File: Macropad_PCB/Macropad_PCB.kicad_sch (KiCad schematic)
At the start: 0 parts

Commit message: Project init
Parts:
- added SW1: SW_Push, Button_Switch_Keyboard:SW_Cherry_MX_1.00u_PCB, symbol Switch:SW_Push
- added SW2: RotaryEncoder, Rotary_Encoder:RotaryEncoder_Alps_EC11E-Switch_Vertical_H20mm, symbol Device:RotaryEncoder
- added U1: MOUDLE-SEEEDUINO-XIAO, footprints:XIAO-Generic-Hybrid-14P-2.54-21X17.8MM, symbol XIAO_RP2040:MOUDLE-SEEEDUINO-XIAO
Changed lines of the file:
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@@
 	(generator_version "9.0")
 	(paper "A4")
+	(symbol
+		(lib_id "Device:RotaryEncoder")
+		(at 157.48 24.13 0)
+		(unit 1)
+		(exclude_from_sim no)
+		(in_bom yes)
+		(on_board yes)
+		(dnp no)
+		(fields_autoplaced yes)
+		(property "Reference" "SW2"
+			(at 163.83 22.8599 0)
+			(effects
+				(font
+					(size 1.27 1.27)
+				)
+				(justify left)
+			)
+		)
+		(property "Value" "RotaryEncoder"
+			(at 163.83 25.3999 0)
+			(effects
+				(font
+					(size 1.27 1.27)
+				)
+				(justify left)
+			)
+		)
+		(property "Footprint" "Rotary_Encoder:RotaryEncoder_Alps_EC11E-Switch_Vertical_H20mm"
+			(at 153.67 20.066 0)
+			(effects
+				(font
+					(size 1.27 1.27)
+				)
+				(hide yes)
+			)
+		)
+		(property "Datasheet" "~"
+			(at 157.48 17.526 0)
+			(effects
+				(font
+					(size 1.27 1.27)
+				)
+				(hide yes)
+			)
+		)
+		(property "Description" "Rotary encoder, dual channel, incremental quadrate outputs"
+			(at 157.48 24.13 0)
+			(effects
+				(font
+					(size 1.27 1.27)
+				)
+				(hide yes)
+			)
+		)
+		(pin "B"
+		)
+		(pin "A"
+		)
+		(pin "C"
+		)
+		(instances
+			(project ""
+				(path "/1a1a6edd-d890-43f8-a81d-660412c01a38"
+					(reference "SW2")
+					(unit 1)
+				)
+			)
+		)
+	)
+	(symbol
+		(lib_id "XIAO_RP2040:MOUDLE-SEEEDUINO-XIAO")
+		(at 74.93 30.48 0)
+		(unit 1)
+		(exclude_from_sim no)
+		(in_bom yes)
+		(on_board yes)
+		(dnp no)
+		(fields_autoplaced yes)
+		(property "Reference" "U1"
+			(at 76.2 15.24 0)
+			(effects
+				(font
+					(size 1.27 1.27)
+				)
+			)
+		)
+		(property "Value" "MOUDLE-SEEEDUINO-XIAO"
+			(at 76.2 17.78 0)
+			(effects
+				(font
+					(size 1.27 1.27)
+				)
+			)
+		)
+		(property "Footprint" "footprints:XIAO-Generic-Hybrid-14P-2.54-21X17.8MM"
+			(at 58.42 27.94 0)
+			(effects
+				(font
+					(size 1.27 1.27)
+				)
+				(hide yes)
+			)
+		)
+		(property "Datasheet" ""
+			(at 58.42 27.94 0)
+			(effects
+				(font
+					(size 1.27 1.27)
+				)
+				(hide yes)
+			)
+		)
+		(property "Description" ""
+			(at 74.93 30.48 0)
+			(effects
+				(font
+					(size 1.27 1.27)
+				)
+				(hide yes)
+			)
+		)
+		(pin "10"
+		)
+		(pin "6"
+		)
+		(pin "7"
+		)
+		(pin "4"
+		)
+		(pin "14"
+		)
+		(pin "3"
+		)
+		(pin "5"
+		)
+		(pin "9"
+		)
+		(pin "8"
+		)
+		(pin "2"
+		)
+		(pin "12"
+		)
+		(pin "11"
+		)
+		(pin "1"
+		)
+		(pin "13"
+		)
+		(instances
+			(project ""
+				(path "/1a1a6edd-d890-43f8-a81d-660412c01a38"
+					(reference "U1")
+					(unit 1)
+				)
+			)
+		)
+	)
+	(symbol
+		(lib_id "Switch:SW_Push")
+		(at 92.71 69.85 0)
+		(unit 1)
+		(exclude_from_sim no)
+		(in_bom yes)
+		(on_board yes)
+		(dnp no)
+		(fields_autoplaced yes)
+		(property "Reference" "SW1"
+			(at 92.71 62.23 0)
+			(effects
+				(font
+					(size 1.27 1.27)
+				)
+			)
+		)
+		(property "Value" "SW_Push"
+			(at 92.71 64.77 0)
+			(effects
+				(font
+					(size 1.27 1.27)
+				)
+			)
+		)
+		(property "Footprint" "Button_Switch_Keyboard:SW_Cherry_MX_1.00u_PCB"
+			(at 92.71 64.77 0)
+			(effects
+				(font
+					(size 1.27 1.27)
+				)
+				(hide yes)
+			)
+		)
+		(property "Datasheet" "~"
+			(at 92.71 64.77 0)
+			(effects
+				(font
+					(size 1.27 1.27)
+				)
+				(hide yes)
+			)
+		)
+		(property "Description" "Push button switch, generic, two pins"
+			(at 92.71 69.85 0)
+			(effects
+				(font
+					(size 1.27 1.27)
+				)
+				(hide yes)
+			)
+		)
+		(pin "1"
+		)
+		(pin "2"
+		)
+		(instances
+			(project ""
+				(path "/1a1a6edd-d890-43f8-a81d-660412c01a38"
+					(reference "SW1")
+					(unit 1)
+				)
+			)
+		)
+	)
 	(sheet_instances
 		(path "/"

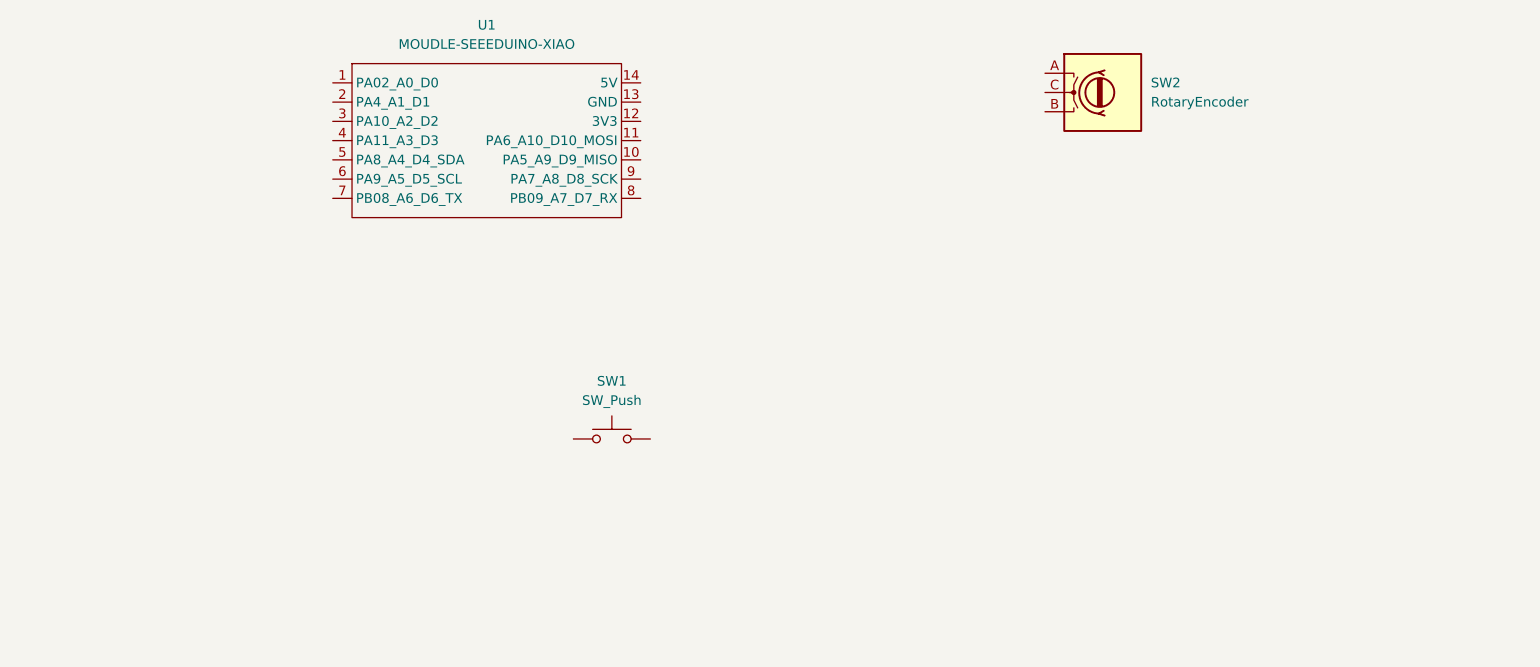
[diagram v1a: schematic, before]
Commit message: Inizio PCB
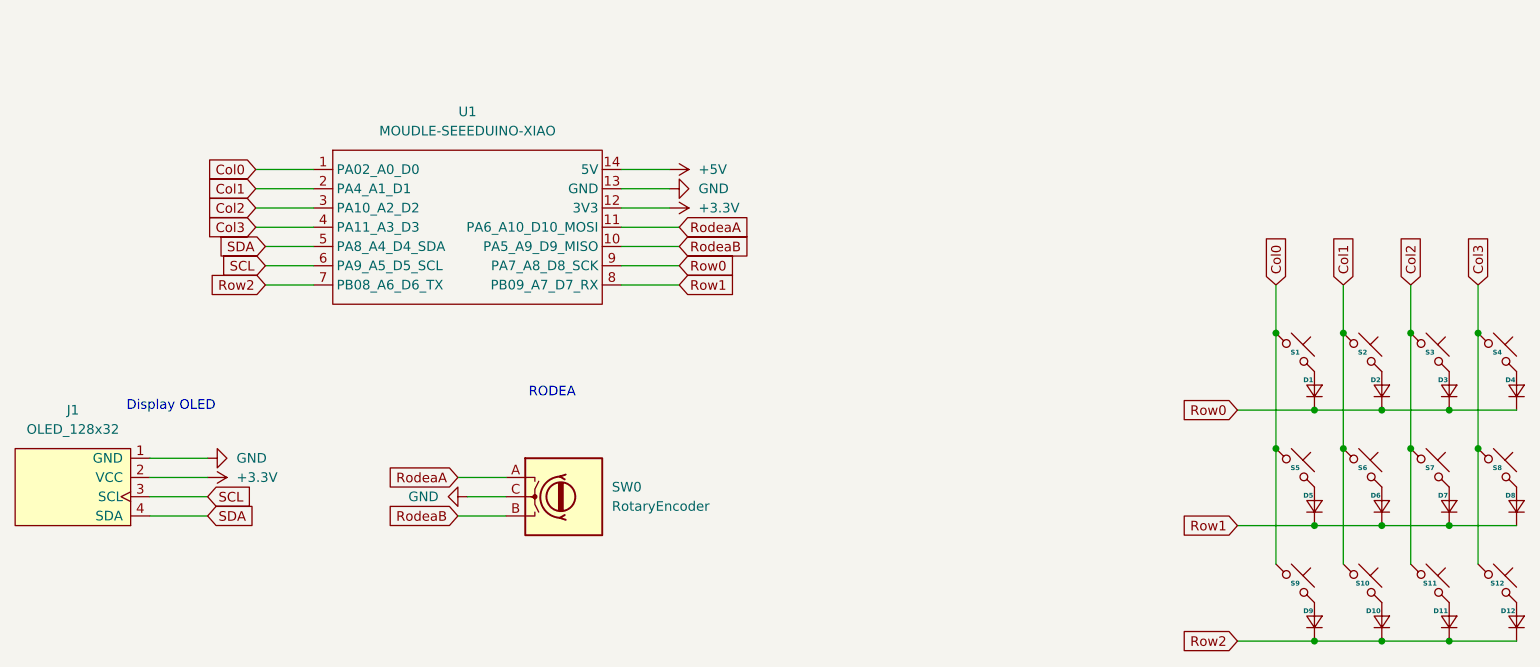
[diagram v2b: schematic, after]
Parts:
- removed SW1: SW_Push, Button_Switch_Keyboard:SW_Cherry_MX_1.00u_PCB, symbol Switch:SW_Push
- added D1, D10, D11, D12, D2, D3, D4, D5, D6, D7, D8, D9: ~, ScottoKeebs_Components:Diode_DO-35, symbol ScottoKeebs:Placeholder_Diode
- added J1: OLED_128x32, ScottoKeebs_Components:OLED_128x32, symbol ScottoKeebs:OLED_128x32
- added S1, S10, S11, S12, S2, S3, S4, S5, S6, S7, S8, S9: ~, ScottoKeebs_MX:MX_PCB_1.00u, symbol ScottoKeebs:Placeholder_Keyswitch
- renumbered SW2 to SW0
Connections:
- net RodeaA: now reaches SW0.A
- net RodeaA: now also U1.11 (PA6_A10_D10_MOSI)
- net RodeaB: now reaches SW0.B
- net RodeaB: now also U1.10 (PA5_A9_D9_MISO)
- net GND: now reaches SW0.C
- net GND: now also U1.13 (GND), J1.1 (GND)
- net Col0: now reaches U1.1 (PA02_A0_D0)
- net Col0: now also S1.1, S5.1, S9.1
- net +3.3V: now reaches U1.12 (3V3)
- net +3.3V: now also J1.2 (VCC)
- net +5V: now reaches U1.14 (5V)
- net Col1: now reaches U1.2 (PA4_A1_D1)
- net Col1: now also S10.1, S2.1, S6.1
- net Col2: now reaches U1.3 (PA10_A2_D2)
- net Col2: now also S11.1, S3.1, S7.1
- net Col3: now reaches U1.4 (PA11_A3_D3)
- net Col3: now also S12.1, S4.1, S8.1
- net SDA: now reaches U1.5 (PA8_A4_D4_SDA)
- net SDA: now also J1.4 (SDA)
- net SCL: now reaches U1.6 (PA9_A5_D5_SCL)
- net SCL: now also J1.3 (SCL)
- net Row2: now reaches U1.7 (PB08_A6_D6_TX)
- net Row2: now also D10.1 (K), D11.1 (K), D12.1 (K), D9.1 (K)
- net Row1: now reaches U1.8 (PB09_A7_D7_RX)
- net Row1: now also D5.1 (K), D6.1 (K), D7.1 (K), D8.1 (K)
- net Row0: now reaches U1.9 (PA7_A8_D8_SCK)
- net Row0: now also D1.1 (K), D2.1 (K), D3.1 (K), D4.1 (K)
- new net: D12.2 (A), S12.2
- new net: D4.2 (A), S4.2
- new net: D3.2 (A), S3.2
- new net: D2.2 (A), S2.2
- new net: D1.2 (A), S1.2
- new net: D6.2 (A), S6.2
- new net: D11.2 (A), S11.2
- new net: D10.2 (A), S10.2
- new net: D9.2 (A), S9.2
- new net: D7.2 (A), S7.2
- new net: D8.2 (A), S8.2
- new net: D5.2 (A), S5.2
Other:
- note added: "Display OLED"
- note added: "RODEA"
- moved on the sheet: SW0, U1

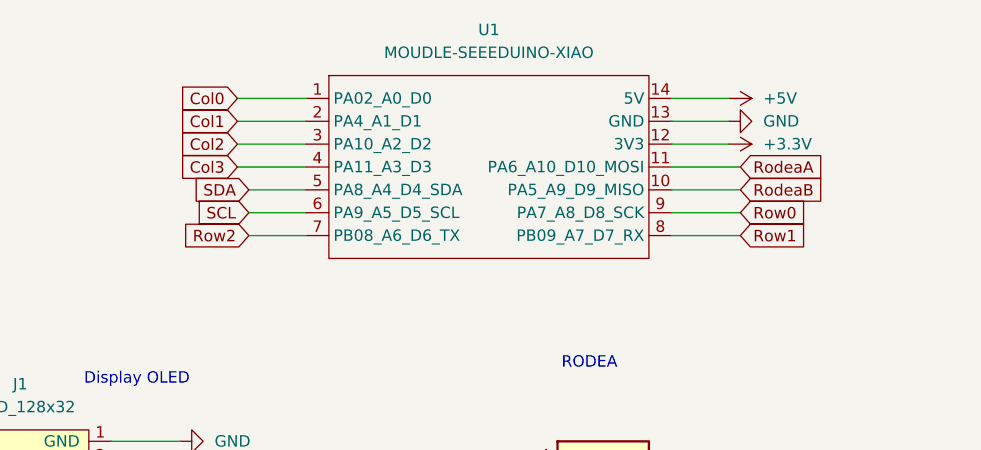
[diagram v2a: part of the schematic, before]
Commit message: PCB. Ancora alcuni errori
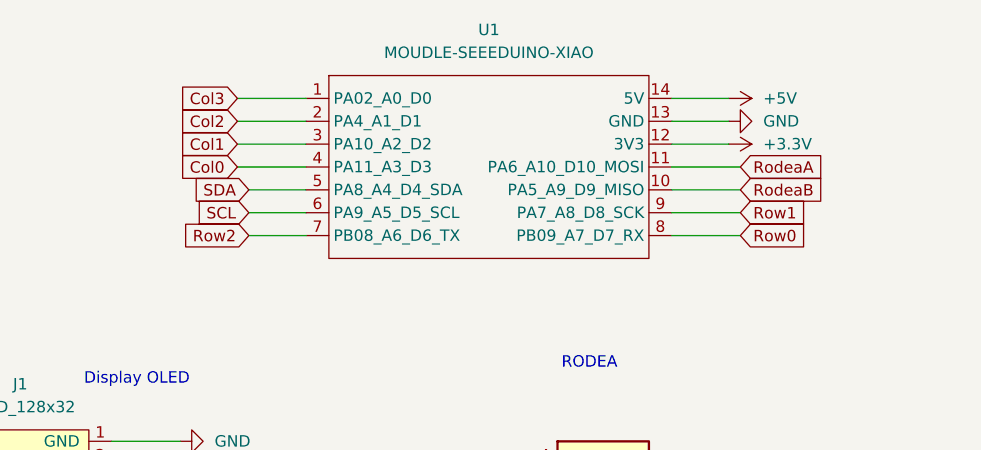
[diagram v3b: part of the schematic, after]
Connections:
- net Col0: now also U1.4 (PA11_A3_D3); no longer U1.1 (PA02_A0_D0)
- net Col1: now also U1.3 (PA10_A2_D2); no longer U1.2 (PA4_A1_D1)
- net Col2: now also U1.2 (PA4_A1_D1); no longer U1.3 (PA10_A2_D2)
- net Col3: now also U1.1 (PA02_A0_D0); no longer U1.4 (PA11_A3_D3)
- net Row0: now also U1.8 (PB09_A7_D7_RX); no longer U1.9 (PA7_A8_D8_SCK)
- net Row1: now also U1.9 (PA7_A8_D8_SCK); no longer U1.8 (PB09_A7_D7_RX)

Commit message: Project exportation
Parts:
- D1, D10, D11, D12, D2, D3, D4, D5, D6, D7, D8, D9: footprint ScottoKeebs_Components:Diode_DO-35 -> Diode_THT:D_DO-35_SOD27_P7.62mm_Horizontal
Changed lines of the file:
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@@
 			)
 		)
-		(property "Footprint" "ScottoKeebs_Components:Diode_DO-35"
+		(property "Footprint" "Diode_THT:D_DO-35_SOD27_P7.62mm_Horizontal"
 			(at 203.2 63.5 90)
 			(effects
@@
 			)
 		)
-		(property "Footprint" "ScottoKeebs_Components:Diode_DO-35"
+		(property "Footprint" "Diode_THT:D_DO-35_SOD27_P7.62mm_Horizontal"
 			(at 185.42 63.5 90)
 			(effects
@@
 			)
 		)
-		(property "Footprint" "ScottoKeebs_Components:Diode_DO-35"
+		(property "Footprint" "Diode_THT:D_DO-35_SOD27_P7.62mm_Horizontal"
 			(at 212.09 63.5 90)
 			(effects
@@
 			)
 		)
-		(property "Footprint" "ScottoKeebs_Components:Diode_DO-35"
+		(property "Footprint" "Diode_THT:D_DO-35_SOD27_P7.62mm_Horizontal"
 			(at 194.31 63.5 90)
 			(effects
@@
 			)
 		)
-		(property "Footprint" "ScottoKeebs_Components:Diode_DO-35"
+		(property "Footprint" "Diode_THT:D_DO-35_SOD27_P7.62mm_Horizontal"
 			(at 203.2 78.74 90)
 			(effects
@@
 			)
 		)
-		(property "Footprint" "ScottoKeebs_Components:Diode_DO-35"
+		(property "Footprint" "Diode_THT:D_DO-35_SOD27_P7.62mm_Horizontal"
 			(at 203.2 93.98 90)
 			(effects
@@
 			)
 		)
-		(property "Footprint" "ScottoKeebs_Components:Diode_DO-35"
+		(property "Footprint" "Diode_THT:D_DO-35_SOD27_P7.62mm_Horizontal"
 			(at 194.31 93.98 90)
 			(effects
@@
 			)
 		)
-		(property "Footprint" "ScottoKeebs_Components:Diode_DO-35"
+		(property "Footprint" "Diode_THT:D_DO-35_SOD27_P7.62mm_Horizontal"
 			(at 212.09 78.74 90)
 			(effects
@@
 			)
 		)
-		(property "Footprint" "ScottoKeebs_Components:Diode_DO-35"
+		(property "Footprint" "Diode_THT:D_DO-35_SOD27_P7.62mm_Horizontal"
 			(at 212.09 93.98 90)
 			(effects
@@
 			)
 		)
-		(property "Footprint" "ScottoKeebs_Components:Diode_DO-35"
+		(property "Footprint" "Diode_THT:D_DO-35_SOD27_P7.62mm_Horizontal"
 			(at 185.42 93.98 90)
 			(effects
@@
 			)
 		)
-		(property "Footprint" "ScottoKeebs_Components:Diode_DO-35"
+		(property "Footprint" "Diode_THT:D_DO-35_SOD27_P7.62mm_Horizontal"
 			(at 194.31 78.74 90)
 			(effects
@@
 			)
 		)
-		(property "Footprint" "ScottoKeebs_Components:Diode_DO-35"
+		(property "Footprint" "Diode_THT:D_DO-35_SOD27_P7.62mm_Horizontal"
 			(at 185.42 78.74 90)
 			(effects
